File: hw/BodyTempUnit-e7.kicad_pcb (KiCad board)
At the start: 4 copper layers, 25 x 30 mm, 27 parts, among them IC1 MAX481CUA, IC2 MEGA8-MI, J1 CONN_IN, J2 CONN_OUT, U1 MAX30205MTA+21-0137I_T833-2-M, U2 LSM6DS3, U3 MCP1801T-3302I_OT

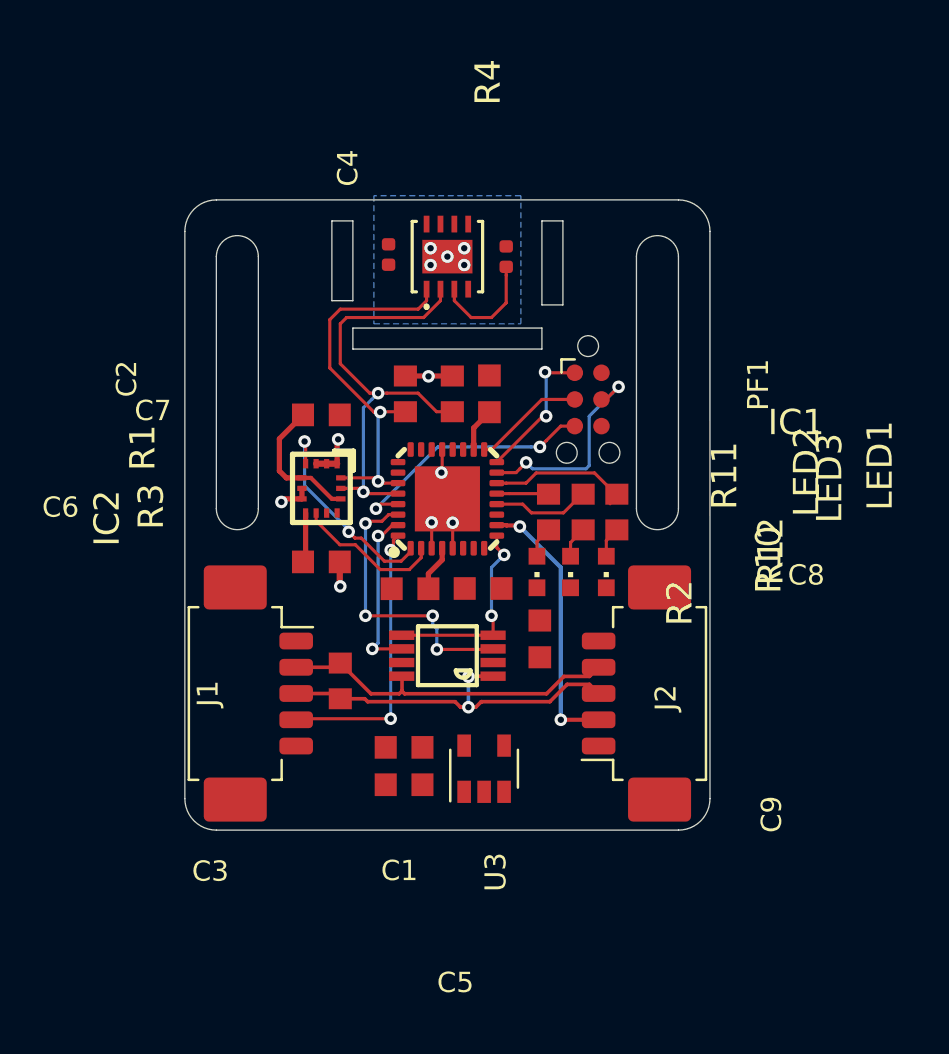
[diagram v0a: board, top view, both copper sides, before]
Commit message: Routing mostly done
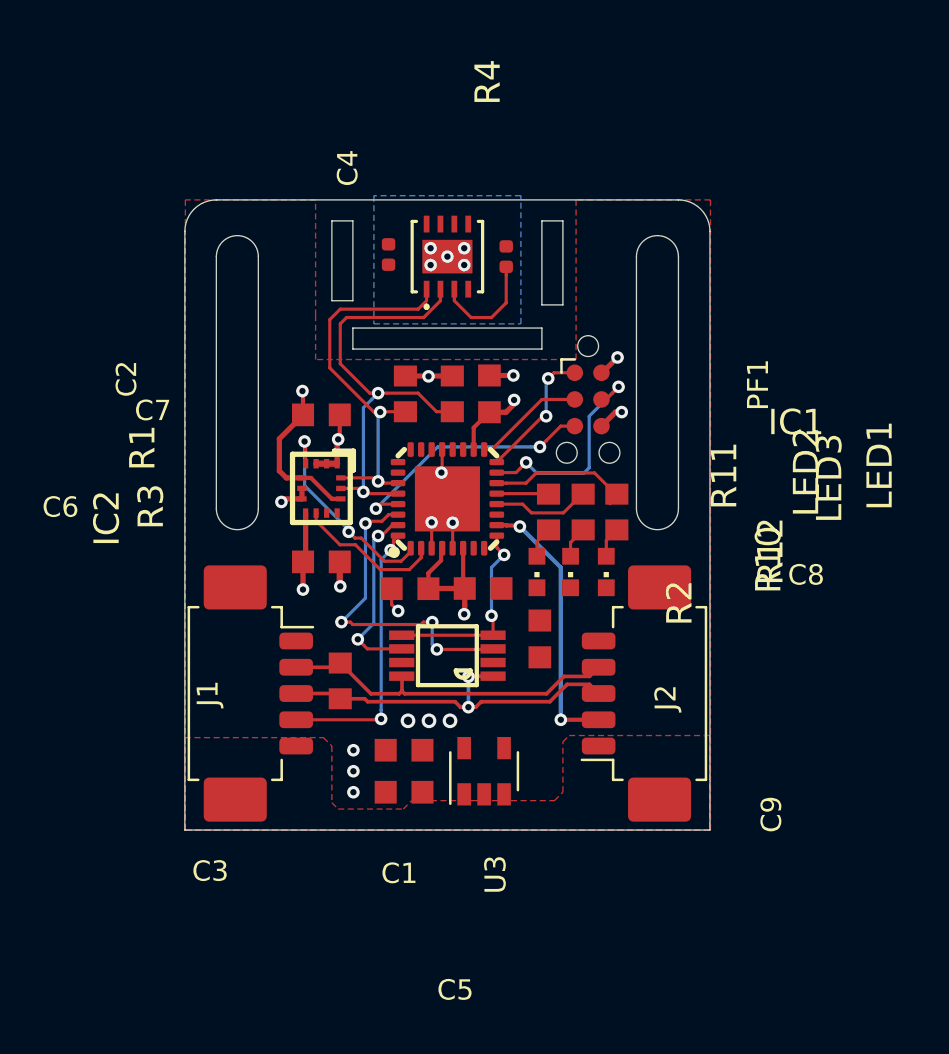
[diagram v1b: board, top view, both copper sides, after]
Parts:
- moved C5 0.36 mm to (75.4, 133.2)
- moved C1 0.14 mm to (75.4, 131.2)
- moved U3 0.12 mm to (79.2, 132.2)
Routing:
- net VCC: track 15.6 -> 25.6 mm, vias 1 -> 9
- net GND: track 12.6 -> 17.4 mm, vias 11 -> 17
- net /RS485_RO: track 13.7 -> 15.4 mm
- net /RS485_DI: track 8.05 -> 8.76 mm
- net /SIG_IN: track 13.7 -> 13.1 mm
- added copper zone on F.Cu, net /VIN
- added copper zone on F.Cu, net GND
- removed copper zone on In2.Cu, net /VIN
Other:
- outline, holes or cut-outs redrawn
- net class Power: trace_width 0.5 -> 0.25
